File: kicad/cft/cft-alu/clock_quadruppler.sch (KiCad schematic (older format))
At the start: 17 parts, among them U11 74HC04, U12 74AC86, U21 74LVC1G04, U46 ICS501

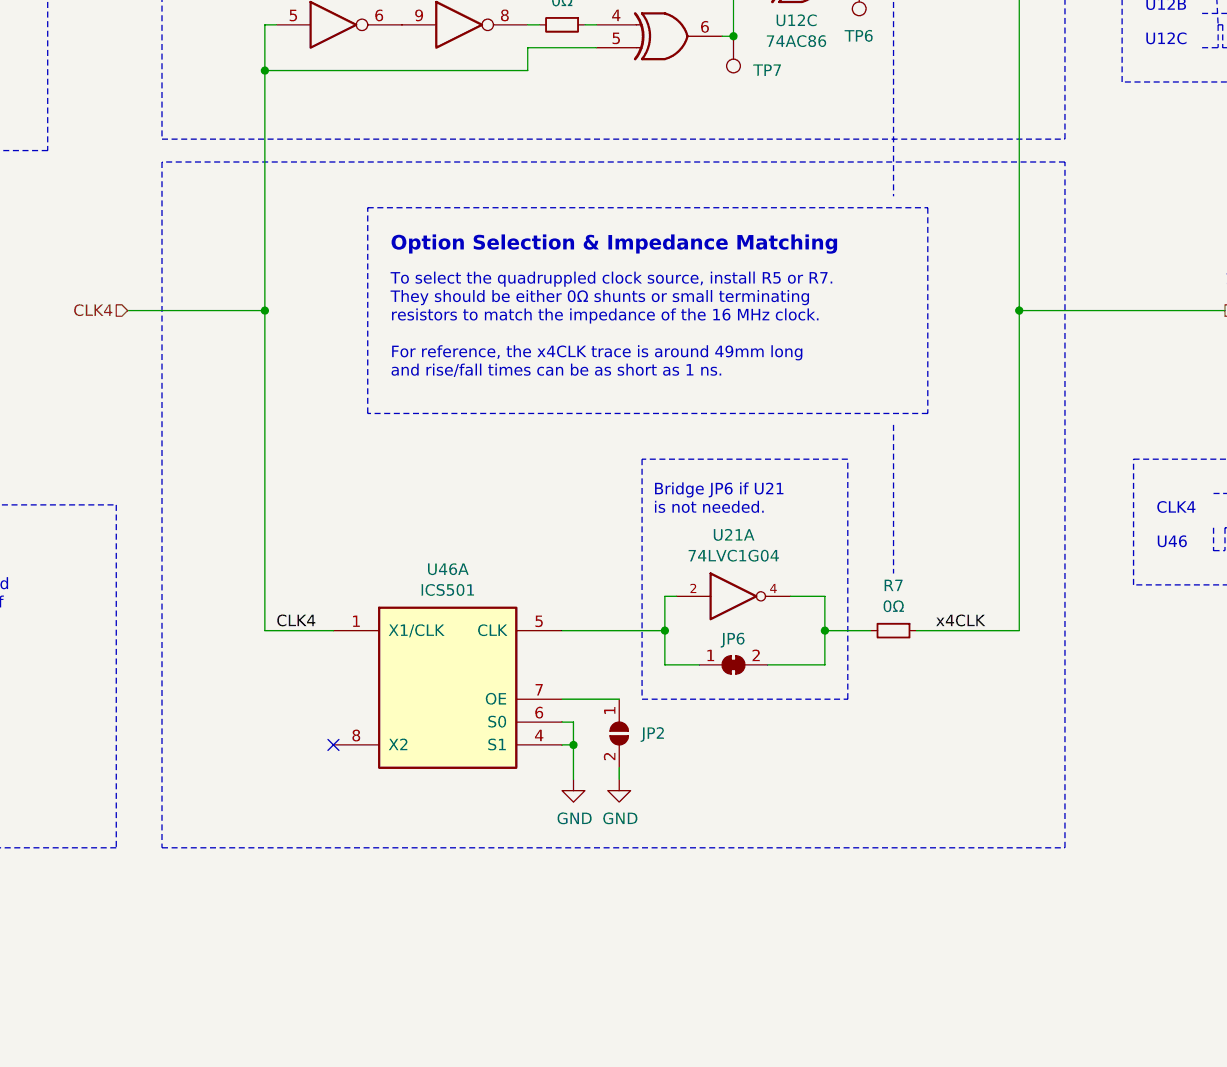
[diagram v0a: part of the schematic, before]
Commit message: Fine-tuning ALU board.
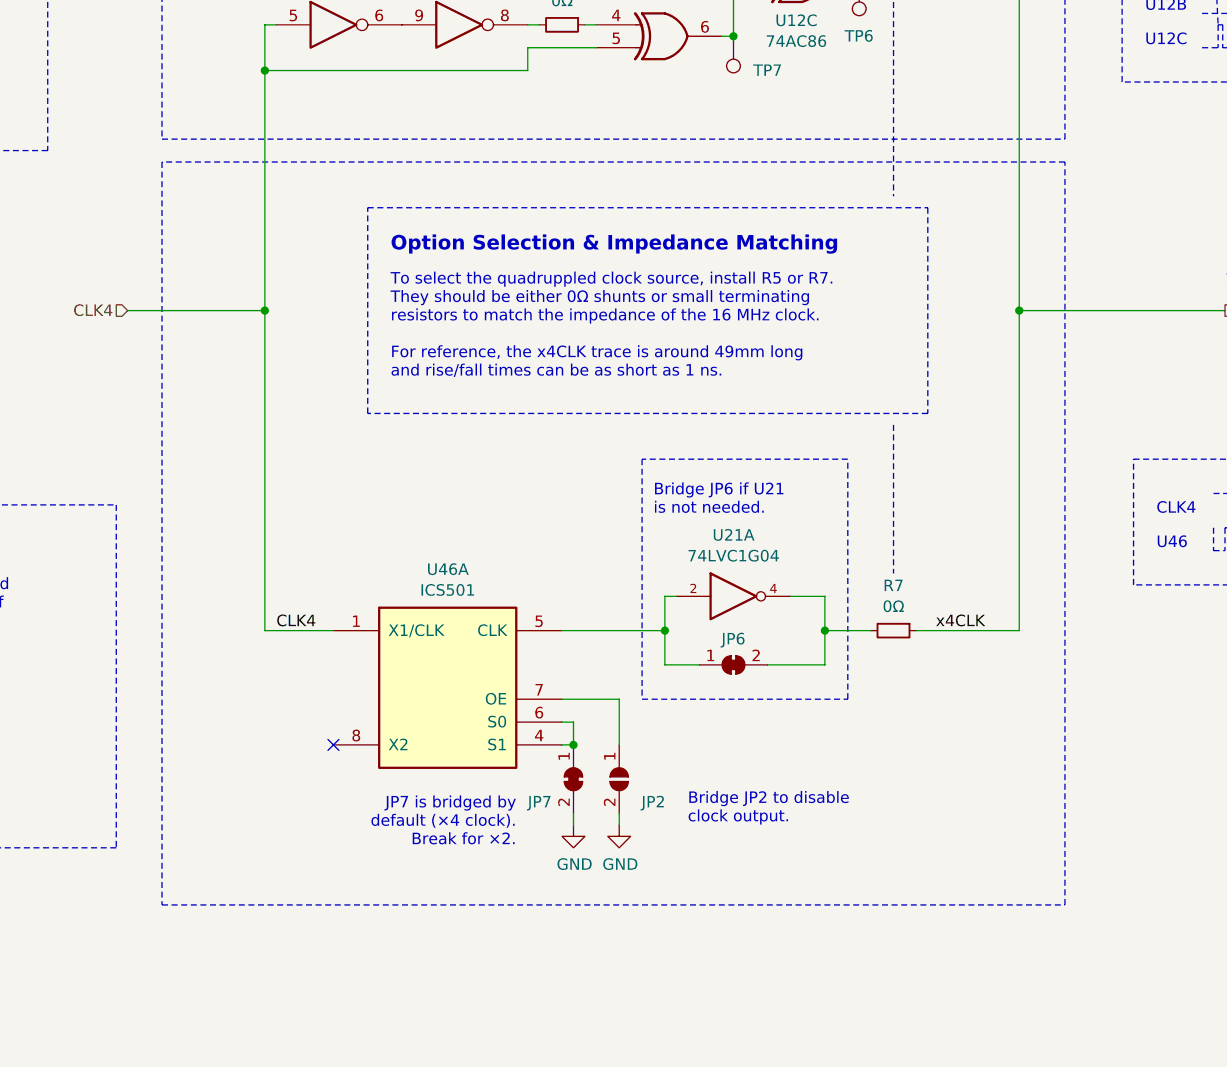
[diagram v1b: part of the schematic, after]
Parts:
- added JP7: SolderJumper_2_Bridged, alexios:SolderJumper-2_P1.3mm_Bridged_RoundedPad1.0x1.5mm, symbol Jumper:SolderJumper_2_Bridged
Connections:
- net GND: now also JP7.2 (B); no longer U46.4 (S1), U46.6 (S0)
- new net: JP7.1 (A), U46.4 (S1), U46.6 (S0)
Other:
- note added: "Bridge JP2 to disable\nclock output."
- note added: "JP7 is bridged by\ndefault (×4 clock).\nBreak for ×2."
- moved on the sheet: JP2
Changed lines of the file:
@@
 L Jumper:SolderJumper_2_Open JP?
 U 1 1 5F0A252B
-P 6050 4950
+P 6050 5150
 AR Path="/5DF75CDE/5F0A252B" Ref="JP?"  Part="1"
 AR Path="/5DF75CDE/5EF12B5A/5F0A252B" Ref="JP2"  Part="1"
-F 0 "JP2" V 6050 5100 50  0000 C CNN
-F 1 "SolderJumper_2_Open" H 6050 5064 50  0001 C CNN
-F 2 "Jumper:SolderJumper-2_P1.3mm_Open_RoundedPad1.0x1.5mm" H 6050 4950 50  0001 C CNN
-F 3 "~" H 6050 4950 50  0001 C CNN
-	1    6050 4950
+F 0 "JP2" V 6150 5300 50  0000 C CNN
+F 1 "SolderJumper_2_Open" H 6050 5264 50  0001 C CNN
+F 2 "Jumper:SolderJumper-2_P1.3mm_Open_RoundedPad1.0x1.5mm" H 6050 5150 50  0001 C CNN
+F 3 "~" H 6050 5150 50  0001 C CNN
+	1    6050 5150
 	0    1    1    0
 $EndComp
@@
 L power:GND #PWR?
 U 1 1 5F0A2531
-P 5850 5150
+P 5850 5350
 AR Path="/5DF75CDE/5F0A2531" Ref="#PWR?"  Part="1"
 AR Path="/5DF75CDE/5EF12B5A/5F0A2531" Ref="#PWR0156"  Part="1"
-F 0 "#PWR0156" H 5850 4900 50  0001 C CNN
-F 1 "GND" H 5855 4977 50  0000 C CNN
-F 2 "" H 5850 5150 50  0001 C CNN
-F 3 "" H 5850 5150 50  0001 C CNN
-	1    5850 5150
-	1    0    0    -1
-$EndComp
-Wire Wire Line
-	5800 4900 5850 4900
-Wire Wire Line
-	5850 5150 5850 5000
+F 0 "#PWR0156" H 5850 5100 50  0001 C CNN
+F 1 "GND" H 5855 5177 50  0000 C CNN
+F 2 "" H 5850 5350 50  0001 C CNN
+F 3 "" H 5850 5350 50  0001 C CNN
+	1    5850 5350
+	1    0    0    -1
+$EndComp
 Wire Wire Line
 	5800 4800 6050 4800
@@
 L power:GND #PWR?
 U 1 1 5F0A253A
-P 6050 5150
+P 6050 5350
 AR Path="/5DF75CDE/5F0A253A" Ref="#PWR?"  Part="1"
 AR Path="/5DF75CDE/5EF12B5A/5F0A253A" Ref="#PWR0222"  Part="1"
-F 0 "#PWR0222" H 6050 4900 50  0001 C CNN
-F 1 "GND" H 6055 4977 50  0000 C CNN
-F 2 "" H 6050 5150 50  0001 C CNN
-F 3 "" H 6050 5150 50  0001 C CNN
-	1    6050 5150
-	1    0    0    -1
-$EndComp
-Wire Wire Line
-	6050 5100 6050 5150
-Wire Wire Line
-	5800 5000 5850 5000
-Connection ~ 5850 5000
-Wire Wire Line
-	5850 5000 5850 4900
+F 0 "#PWR0222" H 6050 5100 50  0001 C CNN
+F 1 "GND" H 6055 5177 50  0000 C CNN
+F 2 "" H 6050 5350 50  0001 C CNN
+F 3 "" H 6050 5350 50  0001 C CNN
+	1    6050 5350
+	1    0    0    -1
+$EndComp
 Text Label 7650 4500 2    50   ~ 0
 x4CLK
@@
 	8000 800  4050 800
 Wire Notes Line
-	8000 5450 8000 2450
-Wire Notes Line
 	8000 2450 4050 2450
-Wire Notes Line
-	4050 2450 4050 5450
-Wire Notes Line
-	4050 5450 8000 5450
 Wire Notes Line width 20 style solid
 	1250 5450 1250 3950
@@
 	1    0    0    -1
 $EndComp
+Wire Wire Line
+	6050 4800 6050 5000
+Wire Wire Line
+	6050 5300 6050 5350
+Wire Wire Line
+	5800 4900 5850 4900
+Wire Wire Line
+	5850 4900 5850 5000
+Wire Wire Line
+	5800 5000 5850 5000
+Wire Wire Line
+	5850 5300 5850 5350
+Text Notes 5600 5450 2    50   ~ 0
+JP7 is bridged by\ndefault (×4 clock).\nBreak for ×2.
+$Comp
+L Jumper:SolderJumper_2_Bridged JP7
+U 1 1 5F94173F
+P 5850 5150
+F 0 "JP7" V 5950 4950 50  0000 L CNN
+F 1 "SolderJumper_2_Bridged" H 5850 5264 50  0001 C CNN
+F 2 "alexios:SolderJumper-2_P1.3mm_Bridged_RoundedPad1.0x1.5mm" H 5850 5150 50  0001 C CNN
+F 3 "~" H 5850 5150 50  0001 C CNN
+	1    5850 5150
+	0    1    1    0
+$EndComp
+Connection ~ 5850 5000
+Text Notes 6350 5350 0    50   ~ 0
+Bridge JP2 to disable\nclock output.
+Wire Notes Line
+	4050 5700 8000 5700
+Wire Notes Line
+	4050 2450 4050 5700
+Wire Notes Line
+	8000 5700 8000 2450
 $EndSCHEMATC
